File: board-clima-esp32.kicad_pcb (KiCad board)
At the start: 2 copper layers, 64.8 x 39.9 mm, 32 parts, among them IC1 ESP32-S3-WROOM-1-N4, J1 Conn_01x02_Pin, J2 Screw_Terminal_01x03, J3 Conn_01x04_Pin, J4 Conn_01x04_Pin, J5 Conn_01x04_Pin, J6 USB_C_Receptacle, Q1 AO3400A, SW1 RESET, SW2 BOOT, U1 AMS1117-3.3, U2 JZC-32F/C

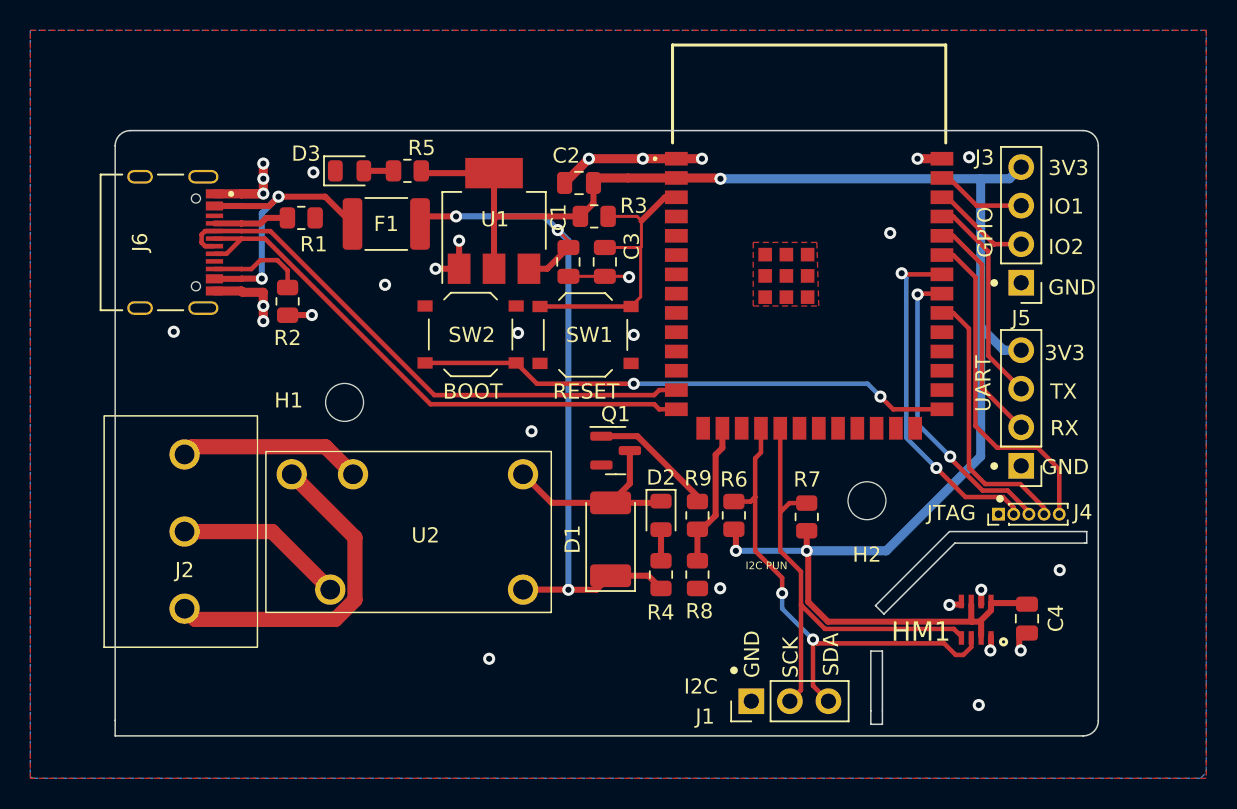
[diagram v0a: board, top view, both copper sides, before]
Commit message: cleanup and some helper in schematic
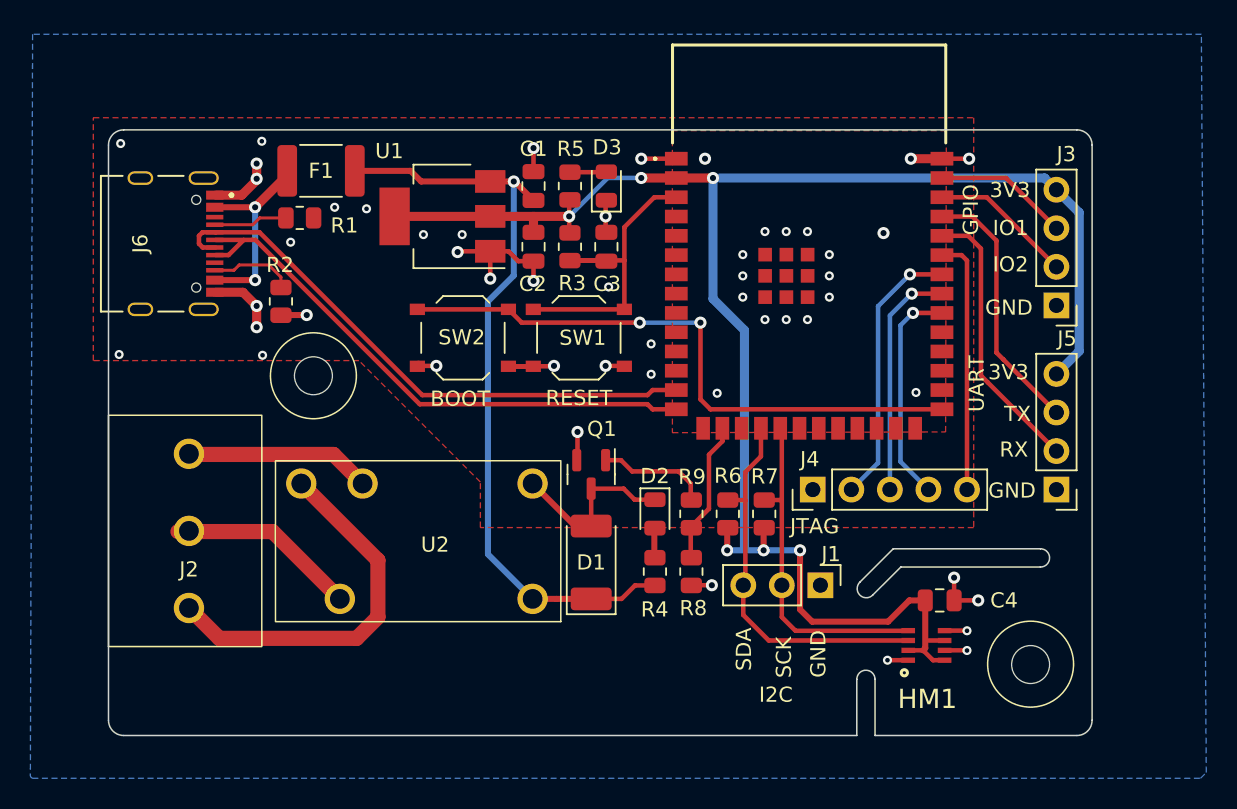
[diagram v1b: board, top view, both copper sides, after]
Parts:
- J4: footprint Connector_PinHeader_1.00mm:PinHeader_1x05_P1.00mm_Vertical -> Connector_PinHeader_2.54mm:PinHeader_1x05_P2.54mm_Vertical
- moved D3 16.9 mm to (123.8, 57.5), turned to 90 degrees
- moved H2 15.3 mm to (151.8, 89.0)
- moved J4 12.3 mm to (137.4, 77.5)
- moved R5 10.8 mm to (121.4, 57.5), turned to 90 degrees
- moved J1 8.89 mm to (137.9, 83.8), turned to -90 degrees
- moved C4 5.87 mm to (145.8, 84.8), turned to 0 degrees
- moved F1 5.54 mm to (105.0, 56.5)
- moved C1 5.50 mm to (119.0, 57.5), turned to 90 degrees
- moved C2 5.16 mm to (119.0, 61.5), turned to -90 degrees
- moved HM1 4.90 mm to (145.9, 88.7), turned to 180 degrees
- moved U1 3.41 mm to (113.0, 59.5), turned to 180 degrees
- moved R7 2.81 mm to (134.2, 79.1)
- moved J3 2.80 mm to (153.4, 77.5)
- moved J5 2.76 mm to (153.4, 65.4)
- moved H1 2.70 mm to (104.5, 70.0)
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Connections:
- J6 pad S1: GND -> unconnected-(J6-SHIELD-PadS1)
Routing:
- net GND: track 35.8 -> 46.3 mm, vias 29 -> 51
- net /SCK: track 32.3 -> 22.5 mm
- net /SDA: track 33.7 -> 25.1 mm, vias 2 -> 0
- net Net-(F1-Pad1): track 19.1 -> 13.3 mm
- net /JTAG_TDI: track 23.1 -> 17.9 mm, vias 2 -> 1
- net /JTAG_TMS: track 22.3 -> 17.3 mm
- net /JTAG_TDO: track 20.1 -> 15.5 mm, vias 2 -> 1
- net /BOOT: track 35.3 -> 39.8 mm
- net /UART_TX: track 13.9 -> 17.6 mm
- net /UART_RX: track 15.2 -> 18.8 mm
- net /GPIO2: track 6.52 -> 9.88 mm
- net /GPIO1: track 5.98 -> 8.91 mm
- net Net-(J2-Pin_1): track 22.1 -> 24.8 mm
- net /JTAG_TCK: track 17.8 -> 15.4 mm, vias 0 -> 1
- net +5V: track 48.0 -> 50.4 mm, vias 3 -> 1
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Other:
- outline, holes or cut-outs redrawn
- board text removed: "I2C PUN"
- board text removed: "JLCJLCJLCJLC"
